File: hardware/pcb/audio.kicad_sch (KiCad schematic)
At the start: 10 parts, among them IC3 TAC5212, J6 PJ-342, J7 PJ-242

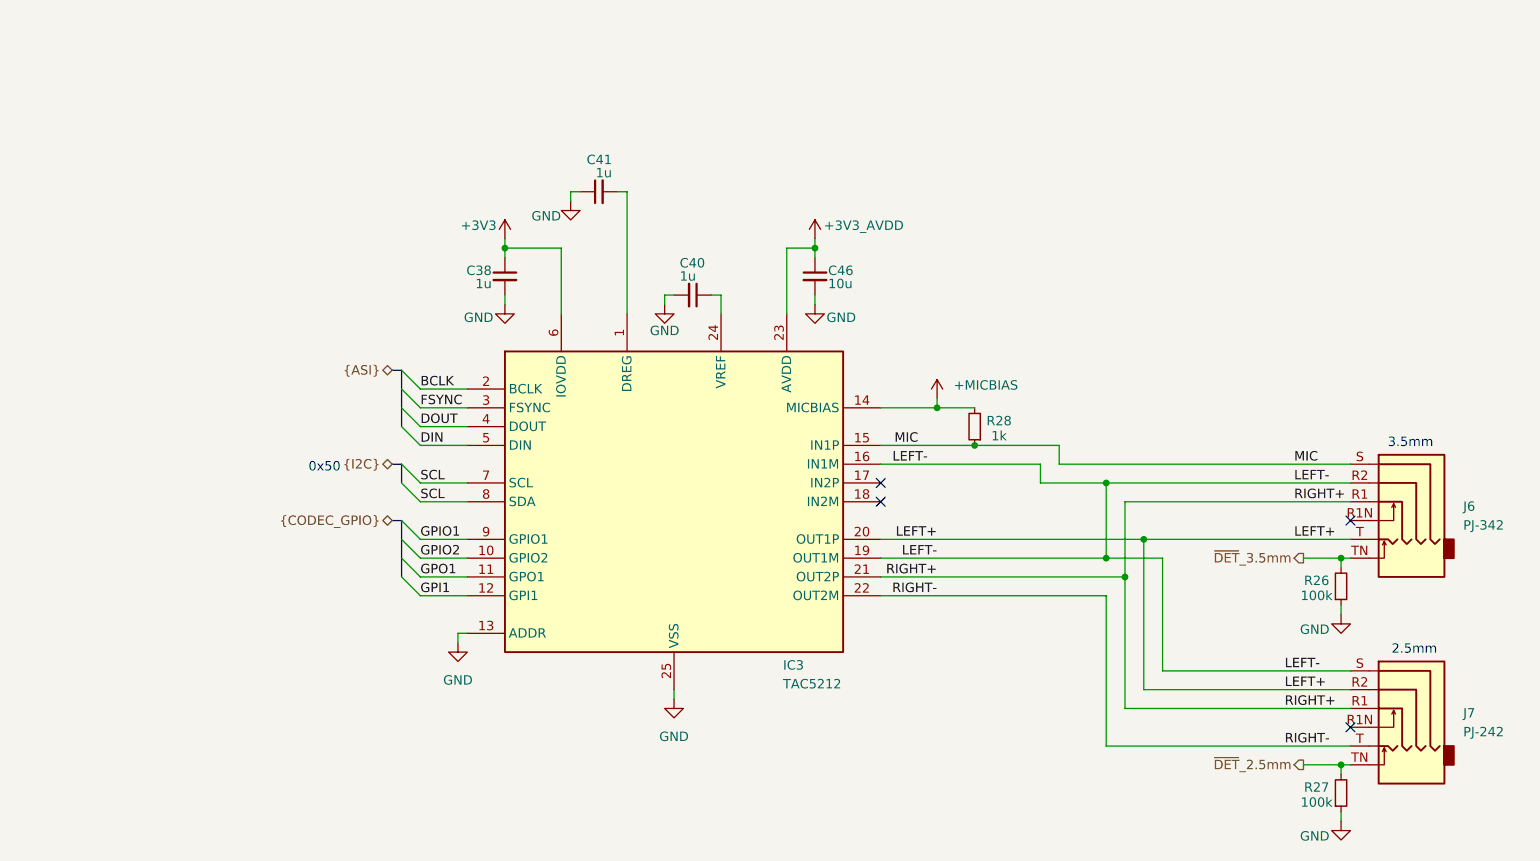
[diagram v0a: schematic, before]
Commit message: looking over stuff, added caps
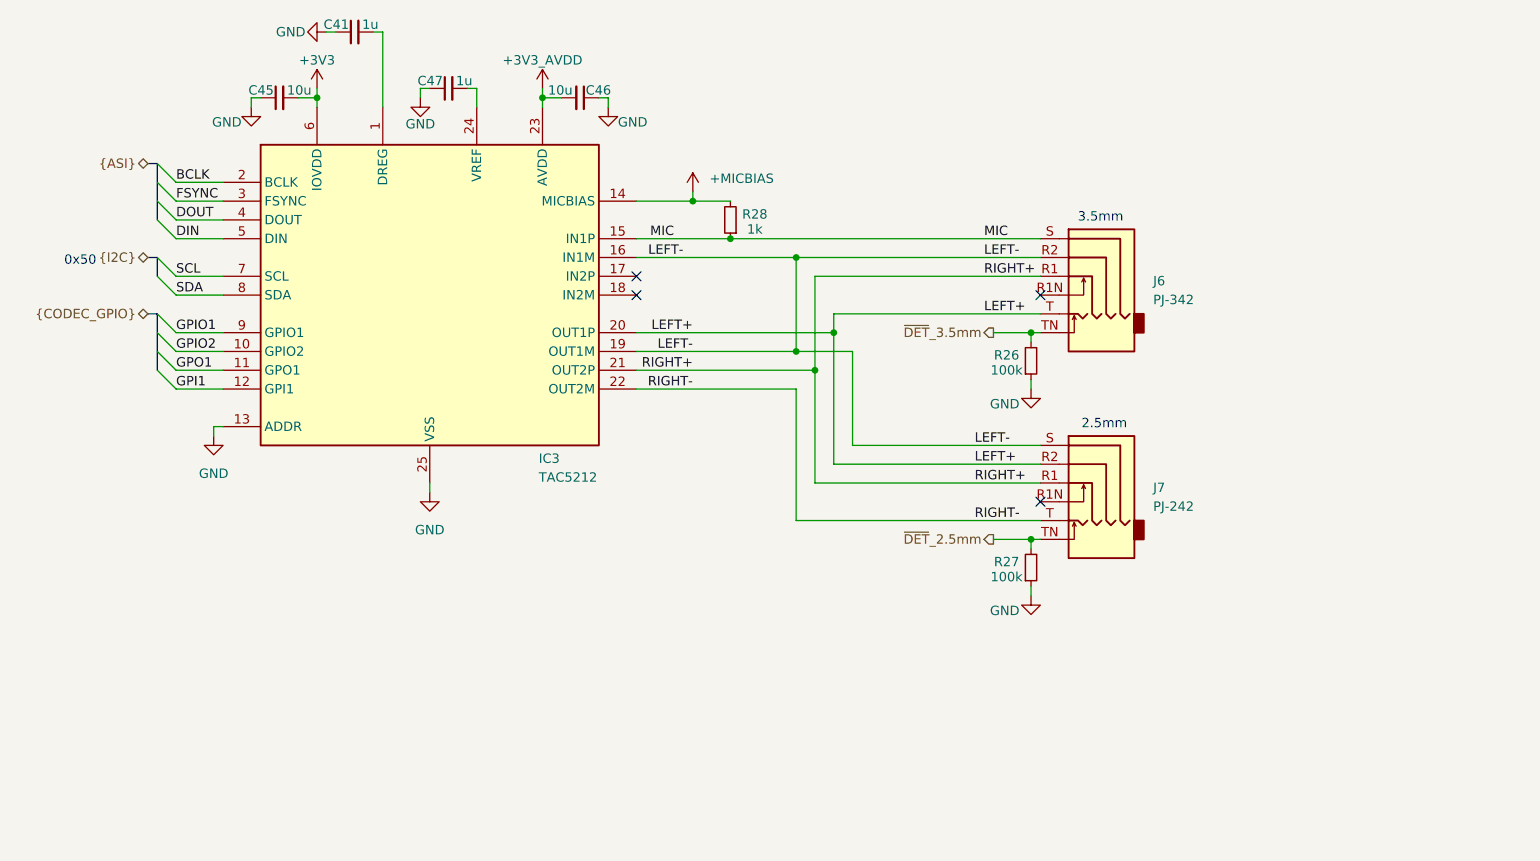
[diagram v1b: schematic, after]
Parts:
- removed C38, C40: 1u, symbol Device:C_Small
- added C45: 10u, Capacitor_SMD:C_0402_1005Metric, symbol Device:C_Small
- added C47: 1u, Capacitor_SMD:C_0402_1005Metric, symbol Device:C_Small
- C41, C46: footprint (none) -> Capacitor_SMD:C_0402_1005Metric
- R26, R27, R28: footprint (none) -> Resistor_SMD:R_0402_1005Metric
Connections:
- net +3V3: now also C45.2
- net +3V3_AVDD: now also C46.2; no longer C46.1
- net GND: now also C46.1, C45.1, C47.1; no longer C46.2
- net SCL: no longer IC3.8 (SDA)
- net at IC3.24 (VREF): now also C47.2
- new net SDA: IC3.8 (SDA)
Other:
- moved on the sheet: C41, IC3, J6, J7, R26, R27, R28
